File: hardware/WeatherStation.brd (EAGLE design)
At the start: 101.3 x 76.2 mm, 9 parts, among them X2 XRJK-S-01-6-4-0-9M2

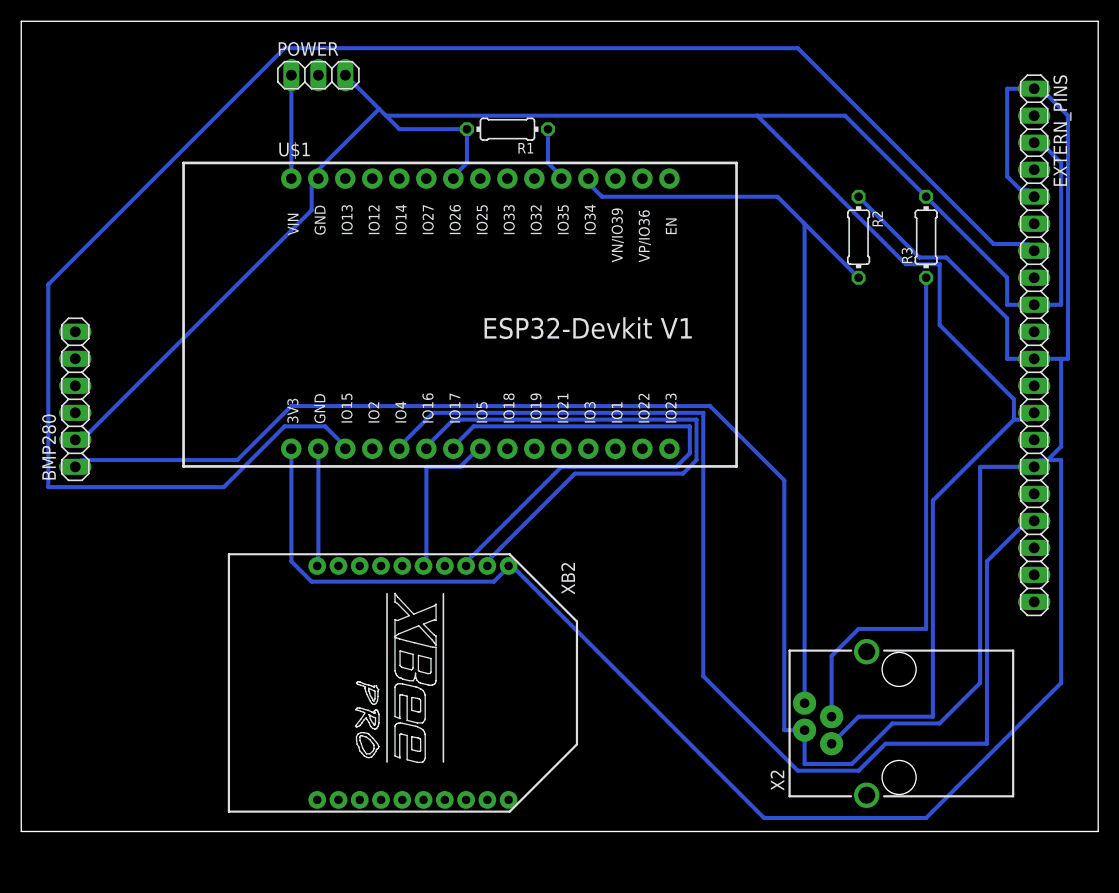
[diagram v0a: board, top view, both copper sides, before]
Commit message: fixing schematic v1.1
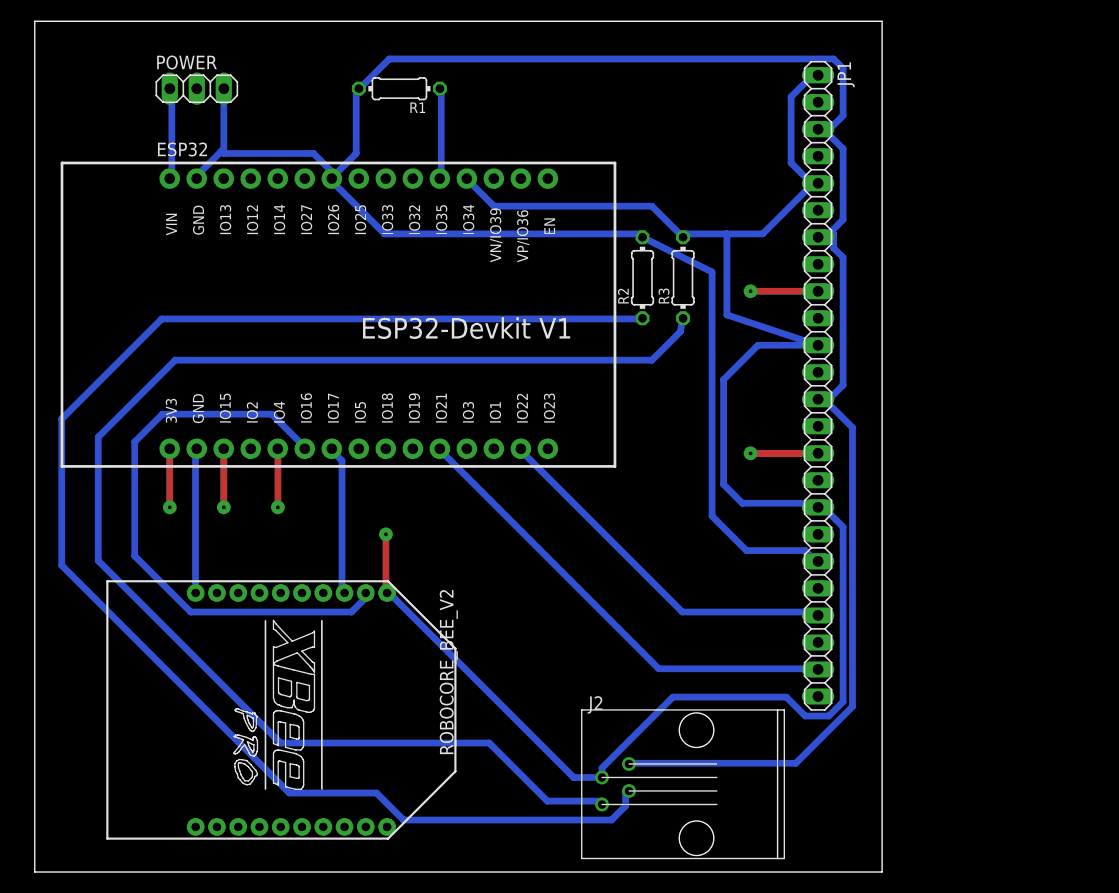
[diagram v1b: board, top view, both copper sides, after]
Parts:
- removed BMP280: (no value), pinhead:1X06
- removed EXTERN_PINS: (no value), pinhead:1X20
- removed U$1: ESP32DEVKITV1, ESP32-DEVKITV1:ESP32-DEVKITV1
- removed X2: XRJK-S-01-6-4-0-9M2, con-xmultiplee:XRJK-S-01-6-4-0-9M2
- removed XB2: XBEE-PRO, maxstream:XBEE-PRO
- added ESP32: ESP32DEVKITV1, ESP32-DEVKITV1:ESP32-DEVKITV1
- added J2: RJ11, con-rj_fixed:RJ11
- added JP1: (no value), pinhead:1X24
- added ROBOCORE_BEE_V2: XBEE-PRO, maxstream:XBEE-PRO
- moved R3 23.2 mm to (61.0, 55.9)
- moved R2 20.7 mm to (57.1, 55.9), turned to 90 degrees
- moved POWER 11.5 mm to (15.2, 73.7)
- moved R1 10.9 mm to (34.3, 73.7)
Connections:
- removed net N$13: U$1.D16, XB2.2
- removed net N$15: U$1.D5, XB2.5
- new net N$9: ESP32.D22, JP1.21
- net N$1: now also ESP32.3V3, ESP32.D34, J2.3, JP1.1, JP1.11, JP1.17, JP1.5, R3.2, ROBOCORE_BEE_V2.1; no longer POWER.1, U$1.VIN
- net N$10: now also ESP32.D21, JP1.23; no longer BMP280.3, U$1.D22
- net N$11: now also ESP32.D17, ROBOCORE_BEE_V2.3; no longer BMP280.4, U$1.D21
- net N$12: now also J2.2, R2.1; no longer U$1.GND@2, XB2.10
- net N$14: now also J2.1, R3.1; no longer U$1.D17, XB2.3
- net N$2: now also ESP32.D26, ESP32.GND@1, J2.4, JP1.13, JP1.19, JP1.3, JP1.7, R2.2; no longer BMP280.2, EXTERN_PINS.13, EXTERN_PINS.3, EXTERN_PINS.9, R3.2, U$1.D26, U$1.GND@1, X2.1
- net N$3: now also ESP32.D35, R1.1; no longer BMP280.1, EXTERN_PINS.1, EXTERN_PINS.11, EXTERN_PINS.15, EXTERN_PINS.5, R2.1, U$1.3V3, X2.2, XB2.1
- net N$4: now also ESP32.D15, JP1.9; no longer R1.1, U$1.D35
- net N$5: now also ESP32.D16, ROBOCORE_BEE_V2.2; no longer EXTERN_PINS.7, U$1.D15
- net N$6: now also ESP32.GND@2, ROBOCORE_BEE_V2.10; no longer EXTERN_PINS.17, U$1.D4
- net N$7: now also ESP32.D4, JP1.15; no longer R2.2, U$1.D34, X2.4
- net N$8: now also ESP32.VIN, POWER.1; no longer R3.1, X2.3
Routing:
- net N$3: track 348.3 -> 8.54 mm
- net N$1: track 9.73 -> 183.1 mm, vias 0 -> 2
- net N$12: track 11.0 -> 137.4 mm
- net N$5: track 160.2 -> 54.1 mm
- net N$6: track 109.4 -> 13.6 mm
- net N$14: track 51.4 -> 128.8 mm
- net N$7: track 74.6 -> 11.9 mm, vias 0 -> 2
- net N$13: track 54.5 -> 0.00 mm
- net N$10: track 0.00 -> 44.2 mm
- net N$8: track 48.7 -> 8.61 mm
- net N$9: track 0.00 -> 34.5 mm
- net N$15: track 15.1 -> 0.00 mm
- net N$11: track 0.00 -> 14.0 mm
- net N$2: track 236.1 -> 245.1 mm
- net N$4: track 5.17 -> 11.9 mm, vias 0 -> 2
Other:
- board size 101.3 x 76.2 mm -> 79.7 x 80 mm
